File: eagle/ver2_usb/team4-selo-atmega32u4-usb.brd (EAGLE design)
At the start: 90 x 40 mm, 35 parts, among them J1 3x2 M, J3 629105136821, SW2 !RESET, U3 ATMEGA32U4-AUR, X2 16 MHz

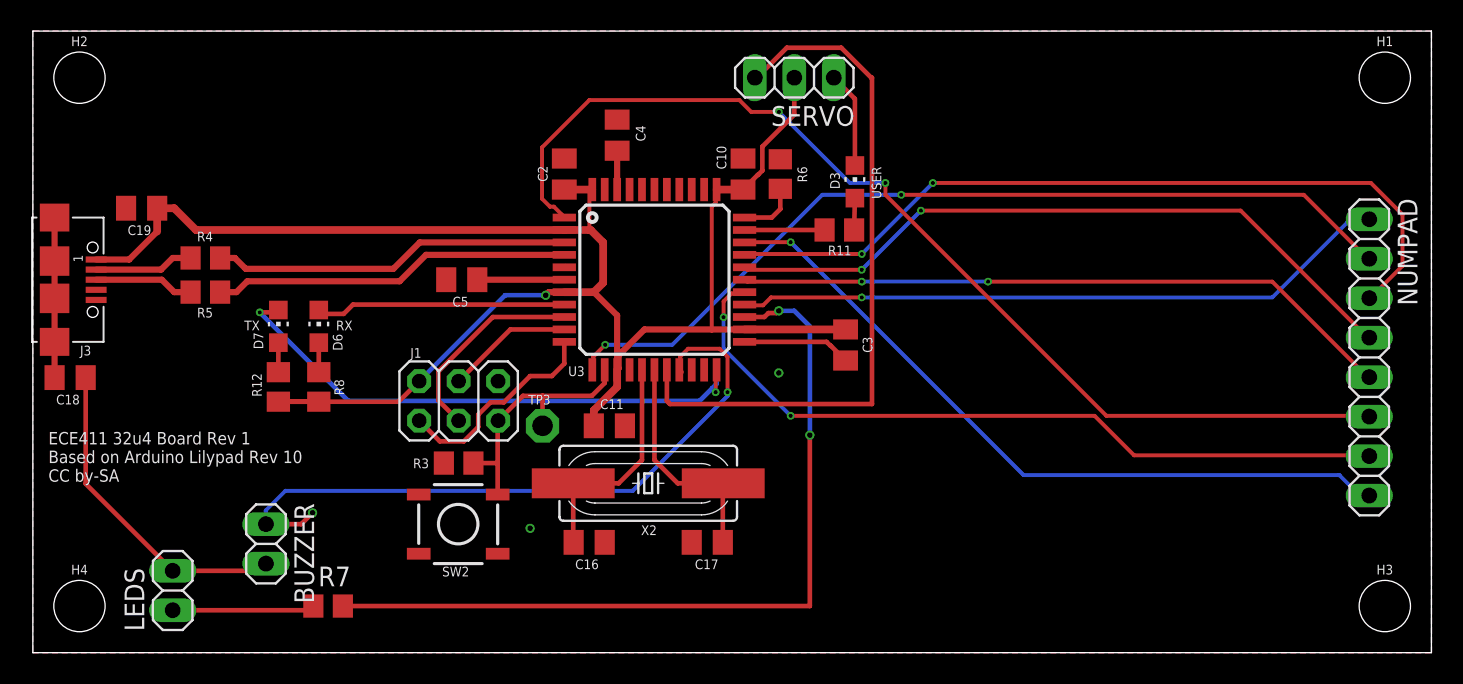
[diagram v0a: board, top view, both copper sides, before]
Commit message: reroute on eagle board, update gitignore
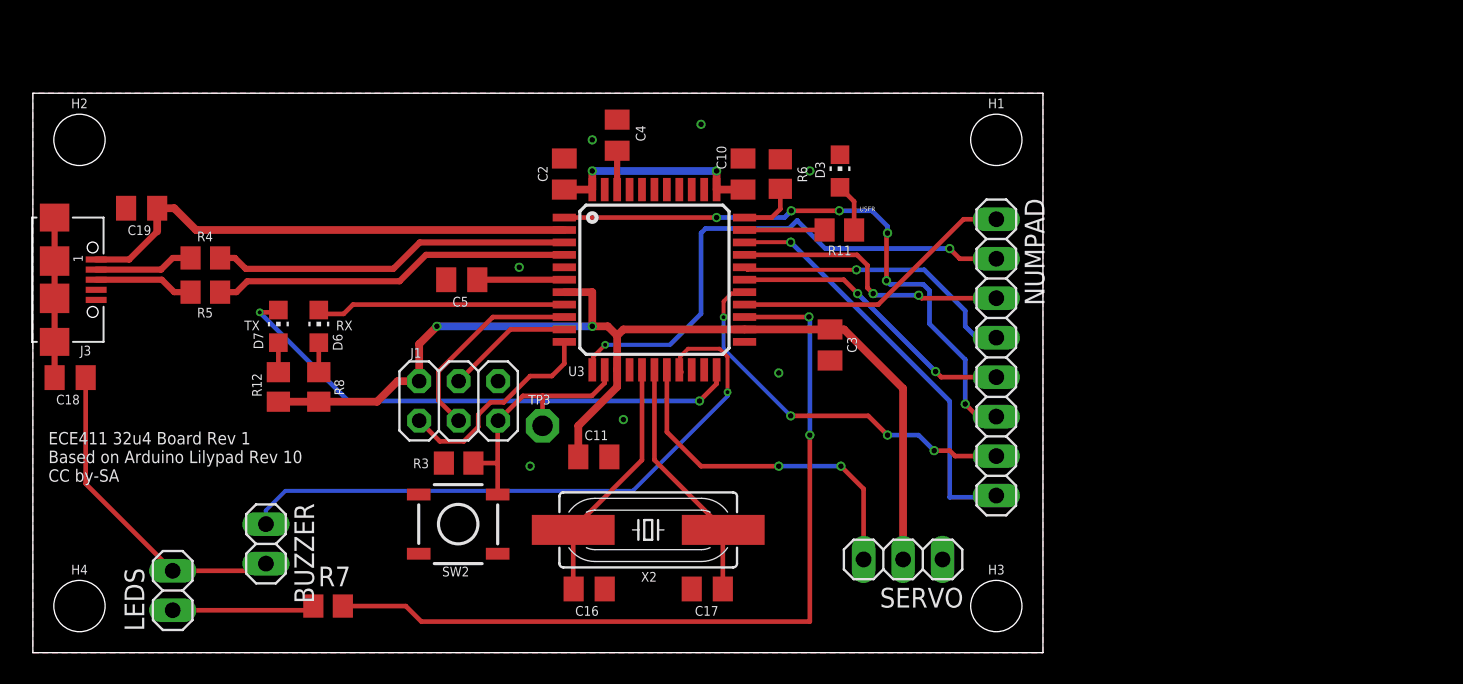
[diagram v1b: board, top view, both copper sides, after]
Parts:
- moved SERVO 31.8 mm to (56.0, 6.00)
- moved H1 25.3 mm to (62.0, 33.0)
- moved H3 25.0 mm to (62.0, 3.00)
- moved NUMPAD 24.0 mm to (62.0, 19.0)
- moved H2 4.00 mm to (3.00, 33.0)
- moved C16 3.00 mm to (35.8, 4.10)
- moved C17 3.00 mm to (43.4, 4.10)
- moved X2 3.00 mm to (39.6, 7.90)
- moved C11 2.24 mm to (36.1, 12.6)
- moved D3 1.18 mm to (51.9, 31.0)
- moved C3 1.00 mm to (51.3, 19.8)
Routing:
- net N$10: track 51.4 -> 18.2 mm
- net N$6: track 68.6 -> 38.5 mm, vias 2 -> 6
- net N$9: track 45.2 -> 18.7 mm, vias 2 -> 1
- net N$12: track 42.5 -> 18.5 mm, vias 1 -> 0
- net N$5: track 49.0 -> 25.1 mm, vias 2 -> 4
- net N$8: track 42.8 -> 18.8 mm
- net N$1: track 45.4 -> 22.7 mm, vias 0 -> 2
- net N$11: track 56.8 -> 34.5 mm
- net N$2: track 46.9 -> 26.7 mm
- net GND: track 34.4 -> 21.2 mm, vias 0 -> 4
- net N$21: track 44.0 -> 40.7 mm, vias 2 -> 1
- net TX_LED: track 36.0 -> 34.4 mm
- net VBUS: track 115.2 -> 116.7 mm, vias 1 -> 4
- net N$17: track 52.8 -> 54.2 mm
- net XTAL2: track 14.7 -> 15.9 mm
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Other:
- board size 90 x 40 mm -> 65 x 36 mm
